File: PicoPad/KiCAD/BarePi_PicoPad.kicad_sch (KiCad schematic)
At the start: 2 parts, among them IC1 Raspberry Pi Pico, J1 OUT

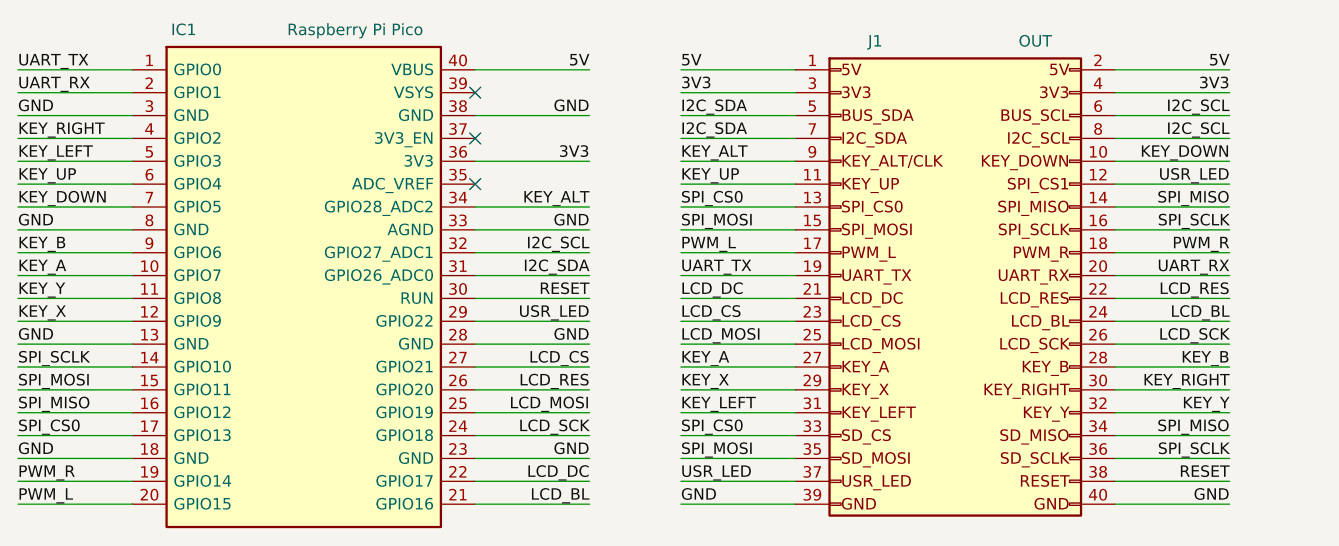
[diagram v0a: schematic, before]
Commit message: init
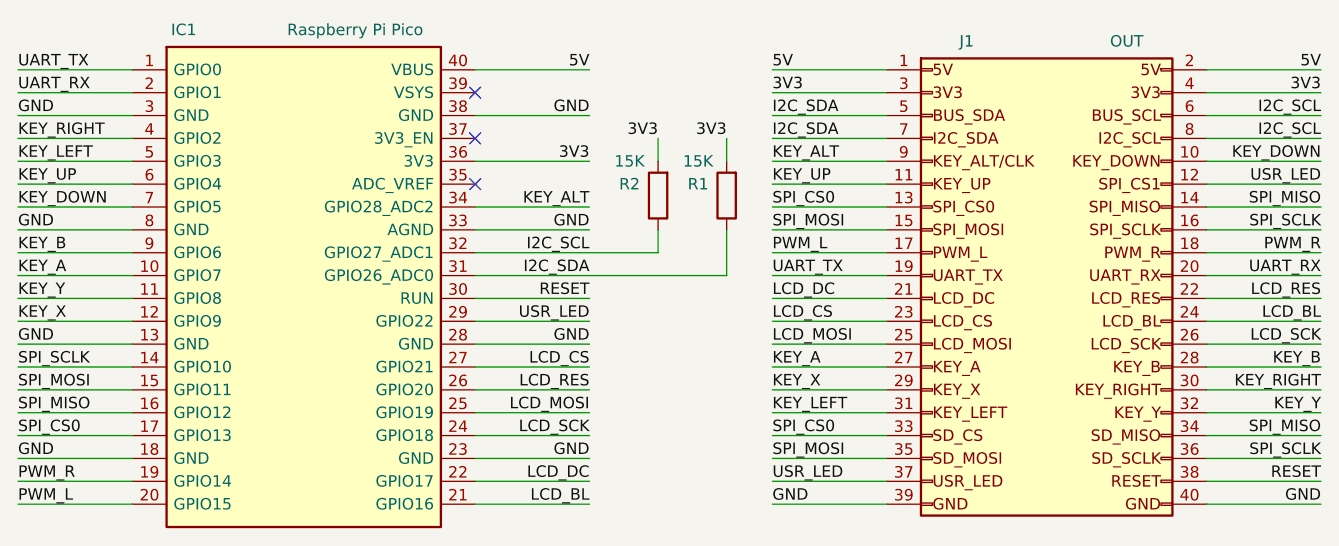
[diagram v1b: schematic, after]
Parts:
- added R1, R2: 15K, Resistor_SMD:R_1206_3216Metric_Pad1.30x1.75mm_HandSolder, symbol Device:R
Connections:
- net 3V3: now also R1.2, R2.2
- net I2C_SCL: now also R2.1
- net I2C_SDA: now also R1.1
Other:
- moved on the sheet: J1
